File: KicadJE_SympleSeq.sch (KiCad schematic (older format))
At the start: 32 parts, among them J101 CV-Out, J102 Reset + Step, J103 CV-G8_Mod1, J104 CV-G8_Mod2, J105 Clk_Hold, J106 G8-Out, J107 Reset + Step 1-4, J108 Reset + Step 5-8, J109 CV-G8_Base, U101 TL082

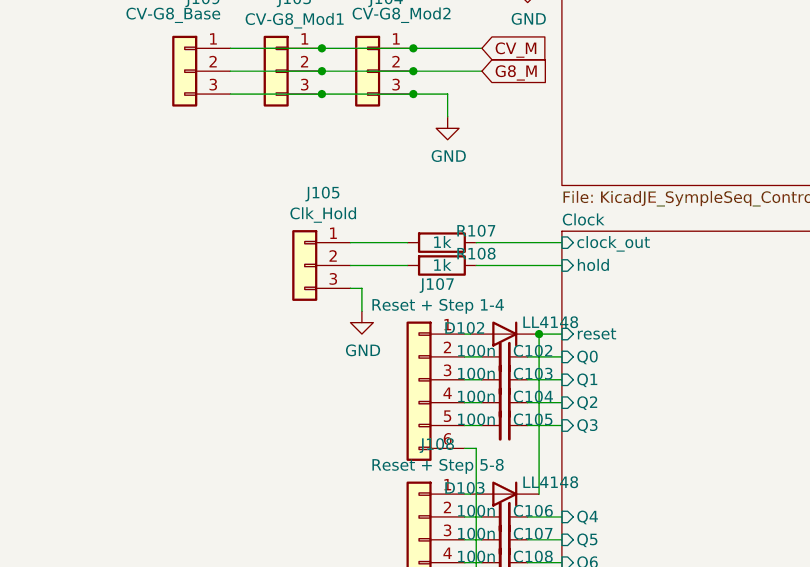
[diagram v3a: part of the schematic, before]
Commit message: hold/rst
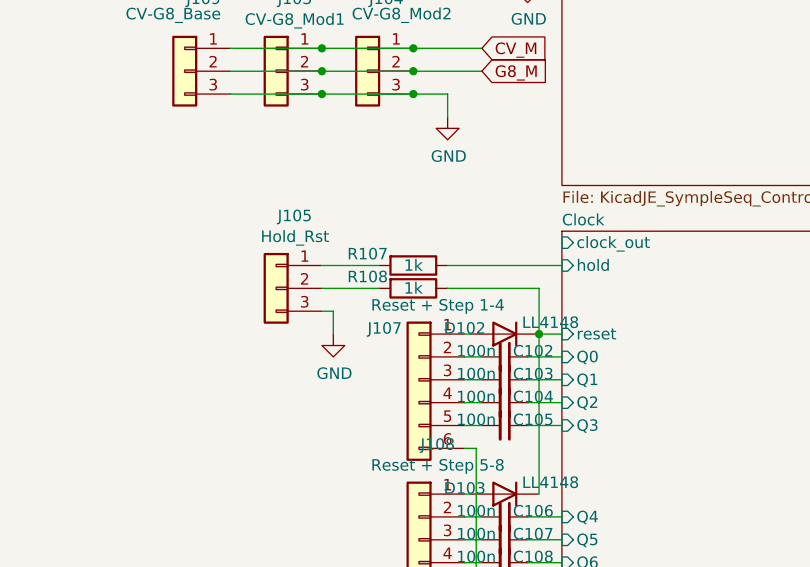
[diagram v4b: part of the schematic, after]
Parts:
- J105: value Clk_Hold -> Hold_Rst
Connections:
- net Clock/clock_out: no longer R107.1
- net Clock/hold: now also R107.1; no longer R108.1
- net Clock/reset: now also R108.1
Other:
- moved on the sheet: J105, R107, R108
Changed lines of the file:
@@
 U 1 1 5DAFAB5F
 P 6375 3800
-F 0 "J107" H 6293 4217 50  0000 C CNN
+F 0 "J107" H 6525 4025 50  0000 C CNN
 F 1 "Reset + Step 1-4" H 6293 4126 50  0000 C CNN
 F 2 "Connector_PinHeader_2.54mm:PinHeader_1x06_P2.54mm_Vertical" H 6375 3800 50  0001 C CNN
@@
 L Connector_Generic:Conn_01x03 J105
 U 1 1 5DB6936A
-P 5875 3300
-F 0 "J105" H 5793 3617 50  0000 C CNN
-F 1 "Clk_Hold" H 5793 3526 50  0000 C CNN
-F 2 "Connector_PinHeader_2.54mm:PinHeader_1x03_P2.54mm_Vertical" H 5875 3300 50  0001 C CNN
-F 3 "~" H 5875 3300 50  0001 C CNN
-	1    5875 3300
+P 5750 3400
+F 0 "J105" H 5668 3717 50  0000 C CNN
+F 1 "Hold_Rst" H 5668 3626 50  0000 C CNN
+F 2 "Connector_PinHeader_2.54mm:PinHeader_1x03_P2.54mm_Vertical" H 5750 3400 50  0001 C CNN
+F 3 "~" H 5750 3400 50  0001 C CNN
+	1    5750 3400
 	-1   0    0    -1
 $EndComp
 Wire Wire Line
-	6075 3300 6325 3300
-Wire Wire Line
-	6075 3200 6325 3200
+	5950 3400 6200 3400
+Wire Wire Line
+	5950 3300 6200 3300
 $Comp
 L Envelope-cache-2018-08-04-13-00-04:GND #PWR0107
 U 1 1 5DB715F6
-P 6125 3500
+P 6000 3600
 AR Path="/5DB715F6" Ref="#PWR0107"  Part="1"
 AR Path="/5C8C5FC0/5DB715F6" Ref="#PWR?"  Part="1"
-F 0 "#PWR0107" H 6125 3250 50  0001 C CNN
-F 1 "GND" H 6130 3327 50  0000 C CNN
-F 2 "" H 6125 3500 50  0001 C CNN
-F 3 "" H 6125 3500 50  0001 C CNN
-	1    6125 3500
-	1    0    0    -1
-$EndComp
-Wire Wire Line
-	6075 3400 6125 3400
-Wire Wire Line
-	6125 3400 6125 3500
+F 0 "#PWR0107" H 6000 3350 50  0001 C CNN
+F 1 "GND" H 6005 3427 50  0000 C CNN
+F 2 "" H 6000 3600 50  0001 C CNN
+F 3 "" H 6000 3600 50  0001 C CNN
+	1    6000 3600
+	1    0    0    -1
+$EndComp
+Wire Wire Line
+	5950 3500 6000 3500
+Wire Wire Line
+	6000 3500 6000 3600
 $Comp
 L Device:R R107
 U 1 1 5DB7317B
-P 6475 3200
+P 6350 3300
 AR Path="/5DB7317B" Ref="R107"  Part="1"
 AR Path="/5C8C5FC0/5DB7317B" Ref="R?"  Part="1"
-F 0 "R107" V 6425 3350 50  0000 C CNN
-F 1 "1k" V 6475 3200 50  0000 C CNN
-F 2 "AJ:R_0805_AJ" V 6405 3200 50  0001 C CNN
-F 3 "~" H 6475 3200 50  0001 C CNN
-	1    6475 3200
+F 0 "R107" V 6300 3100 50  0000 C CNN
+F 1 "1k" V 6350 3300 50  0000 C CNN
+F 2 "AJ:R_0805_AJ" V 6280 3300 50  0001 C CNN
+F 3 "~" H 6350 3300 50  0001 C CNN
+	1    6350 3300
 	0    1    1    0
 $EndComp
@@
 L Device:R R108
 U 1 1 5DB73B0A
-P 6475 3300
+P 6350 3400
 AR Path="/5DB73B0A" Ref="R108"  Part="1"
 AR Path="/5C8C5FC0/5DB73B0A" Ref="R?"  Part="1"
-F 0 "R108" V 6425 3450 50  0000 C CNN
-F 1 "1k" V 6475 3300 50  0000 C CNN
-F 2 "AJ:R_0805_AJ" V 6405 3300 50  0001 C CNN
-F 3 "~" H 6475 3300 50  0001 C CNN
-	1    6475 3300
+F 0 "R108" V 6300 3200 50  0000 C CNN
+F 1 "1k" V 6350 3400 50  0000 C CNN
+F 2 "AJ:R_0805_AJ" V 6280 3400 50  0001 C CNN
+F 3 "~" H 6350 3400 50  0001 C CNN
+	1    6350 3400
 	0    1    1    0
 $EndComp
@@
 Connection ~ 5950 2550
 Wire Wire Line
-	6625 3200 7000 3200
-Wire Wire Line
 	6575 3700 6650 3700
 Wire Wire Line
@@
 Wire Wire Line
 	2300 3600 2350 3600
-Wire Wire Line
-	6625 3300 7000 3300
 $Comp
 L Diode:LL4148 D?
@@
 Wire Wire Line
 	2350 3600 2500 3600
+Wire Wire Line
+	6900 3600 6900 3400
+Wire Wire Line
+	6500 3400 6900 3400
+Wire Wire Line
+	6500 3300 7000 3300
 $EndSCHEMATC
